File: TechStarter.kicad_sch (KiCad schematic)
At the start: 28 parts, among them J1 Conn_01x04_Socket, J10 Conn_01x03_Socket, J11 Conn_01x03_Socket, J12 Conn_01x04_Pin, J2 Conn_01x04_Socket, J5 Conn_01x03_Socket, J7 Conn_01x03_Socket, J8 Conn_01x03_Socket, J9 Conn_01x03_Socket, U1 STM32F446RETx, U2 TMC2209-LA, U3 TMC2209-LA, U5 MX25L3233FM1

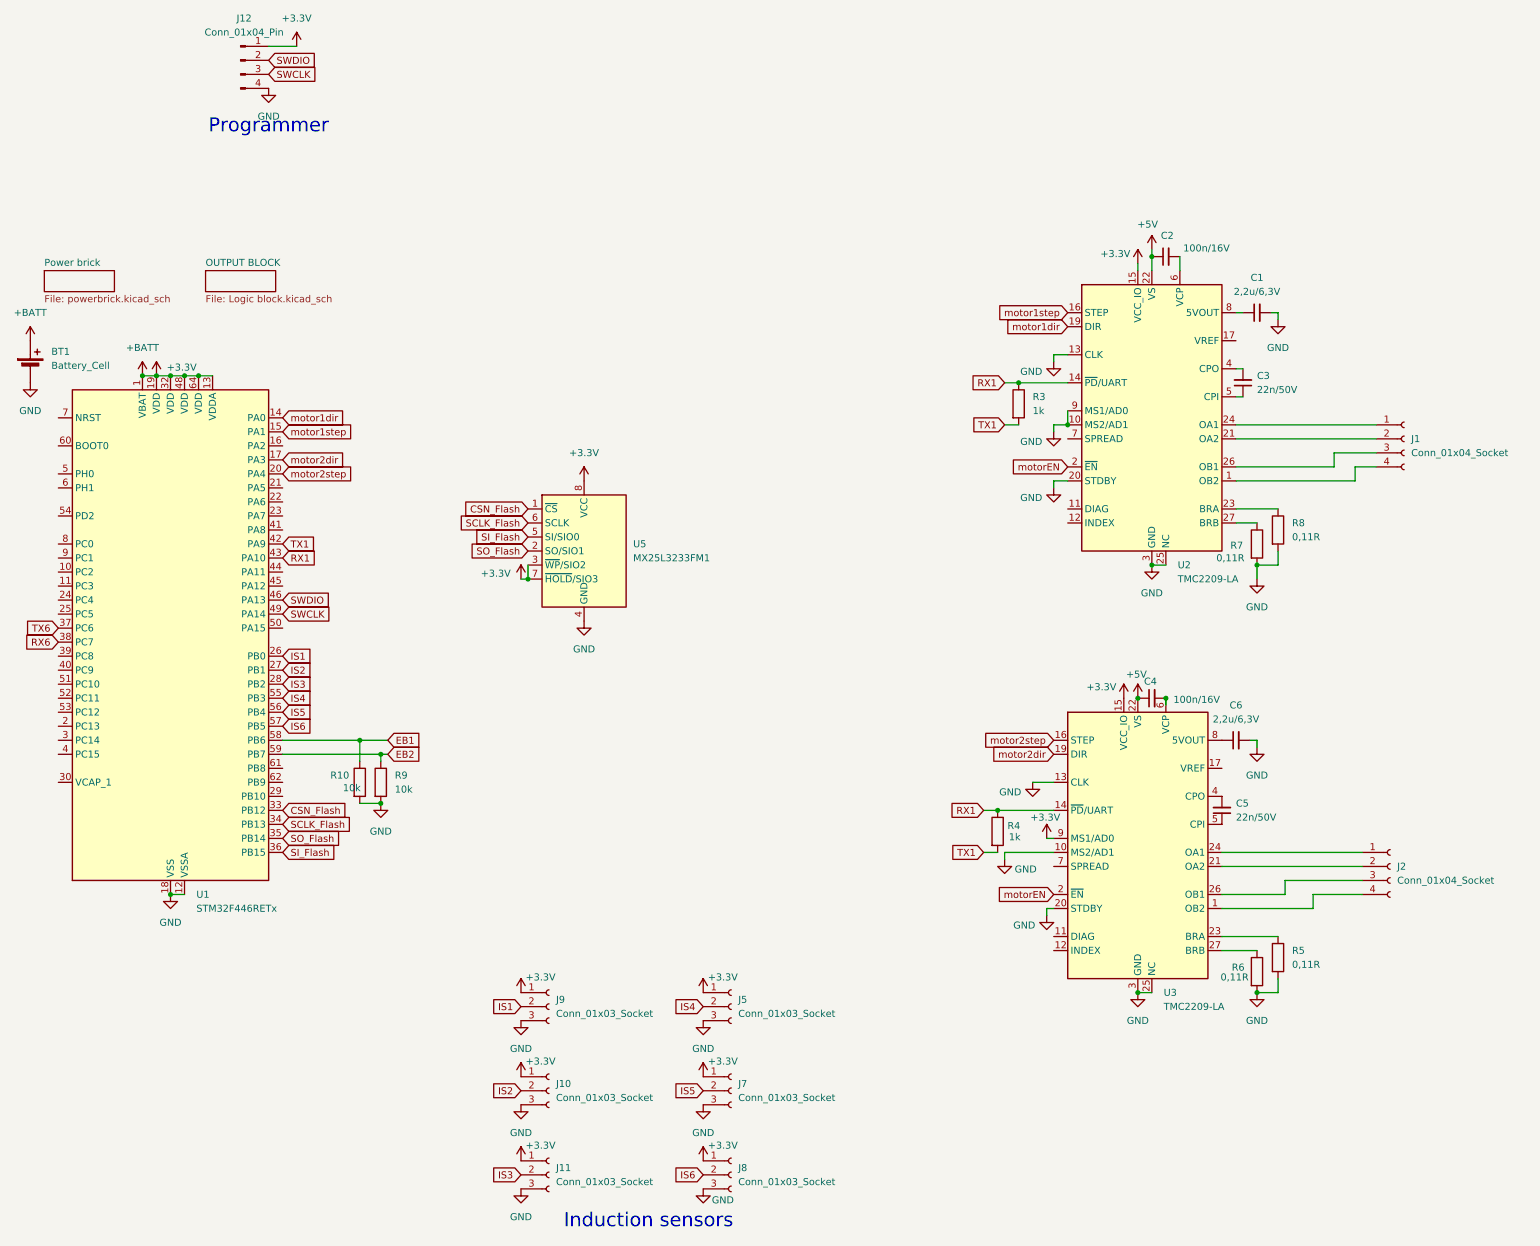
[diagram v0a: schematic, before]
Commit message: Board
started board ...
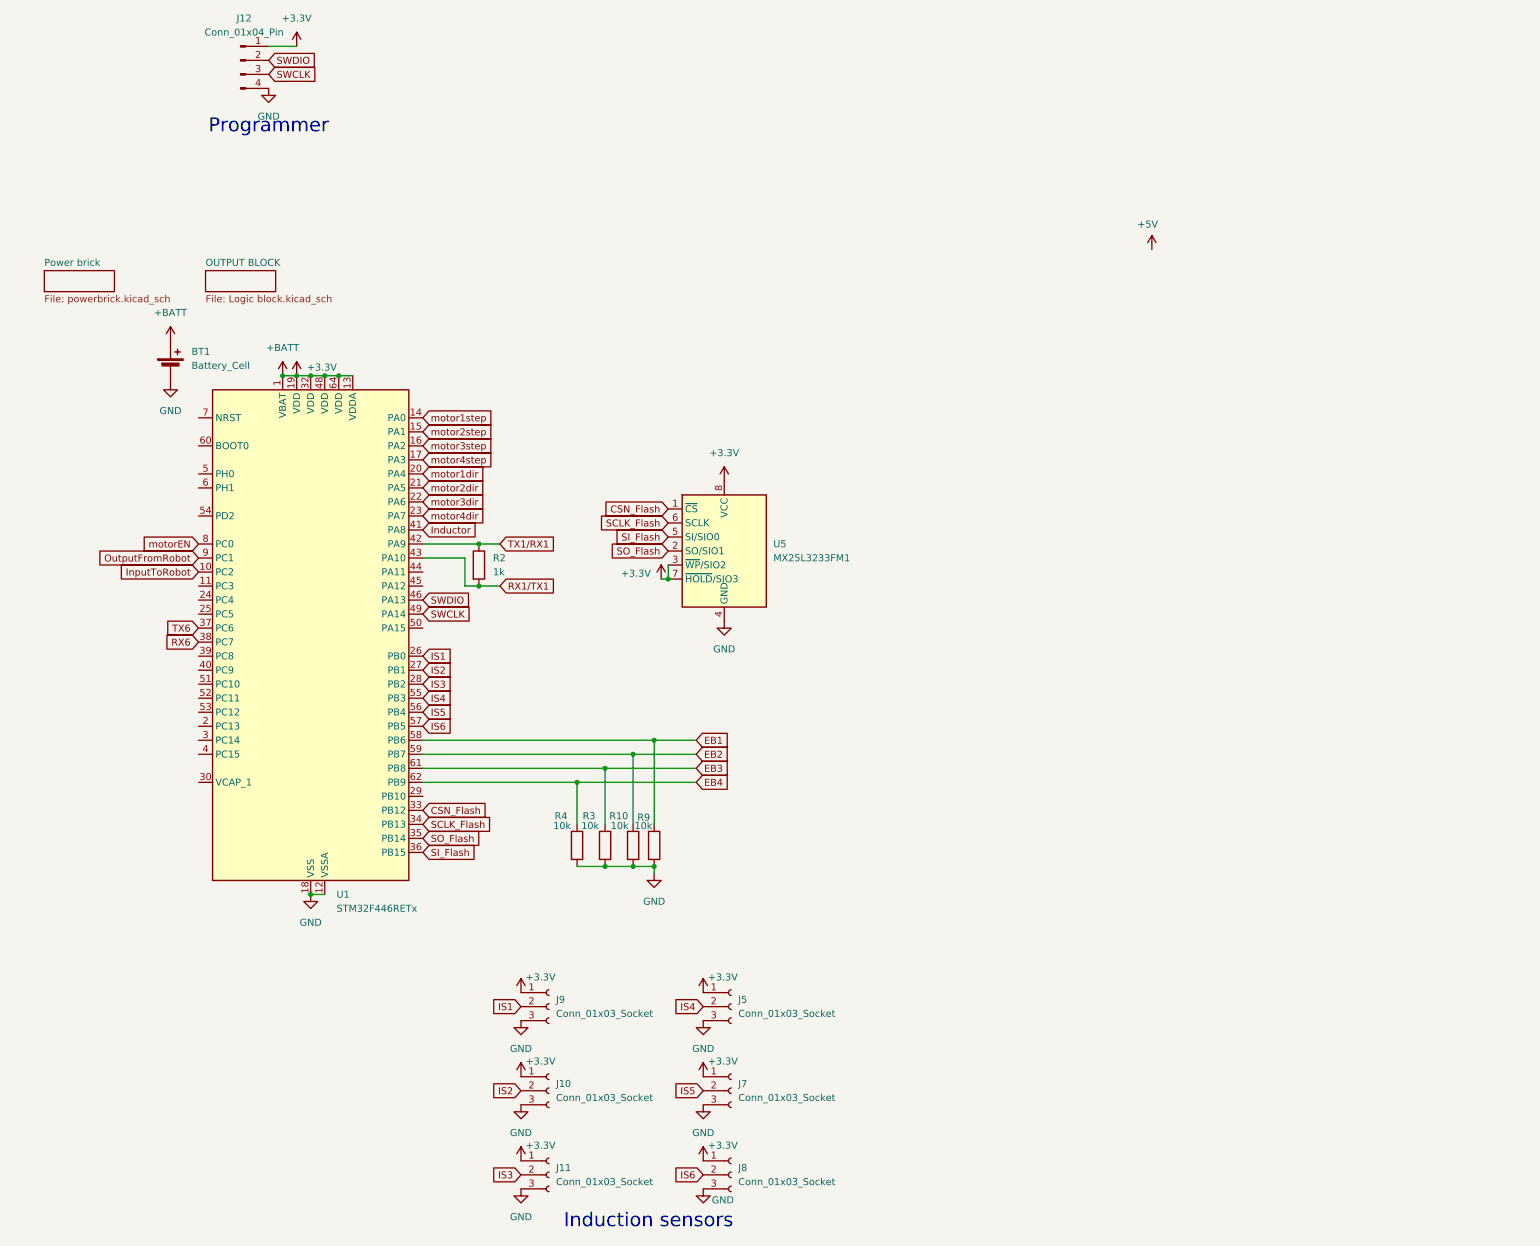
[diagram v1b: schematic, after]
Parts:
- removed C1: 2,2u/6,3V, Connector_JST:JST_XH_S3B-XH-A_1x03_P2.50mm_Horizontal, symbol Device:C_Small
- removed C2, C4: 100n/16V, symbol Device:C_Small
- removed C3, C5: 22n/50V, symbol Device:C_Small
- removed C6: 2,2u/6,3V, symbol Device:C_Small
- removed J1, J2: Conn_01x04_Socket, symbol Connector:Conn_01x04_Socket
- removed R5, R6, R7, R8: 0,11R, symbol Device:R
- removed U2, U3: TMC2209-LA, Package_DFN_QFN:VQFN-28-1EP_5x5mm_P0.5mm_EP3.7x3.7mm_ThermalVias, symbol Driver_Motor:TMC2209-LA
- added R2: 1k, Resistor_SMD:R_0603_1608Metric, symbol Device:R
- R10, R9: footprint (none) -> Resistor_SMD:R_0603_1608Metric
- R3, R4: value 1k -> 10k; footprint (none) -> Resistor_SMD:R_0603_1608Metric
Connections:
- net EB1: now also R9.1; no longer R10.1
- net EB2: now also R10.1; no longer R9.1
- net GND: now also R3.2, R4.2
- net motor1dir: now also U1.20 (PA4); no longer U1.14 (PA0)
- net motor1step: now also U1.14 (PA0); no longer U1.15 (PA1)
- net motor2dir: now also U1.21 (PA5); no longer U1.17 (PA3)
- net motor2step: now also U1.15 (PA1); no longer U1.20 (PA4)
- net motorEN: now also U1.8 (PC0)
- net InputToRobot: now reaches U1.10 (PC2)
- net motor3step: now reaches U1.16 (PA2)
- net motor3dir: now reaches U1.22 (PA6)
- net motor4dir: now reaches U1.23 (PA7)
- net Inductor: now reaches U1.41 (PA8)
- net EB3: now reaches U1.61 (PB8)
- net EB3: now also R3.1
- net EB4: now reaches U1.62 (PB9)
- net EB4: now also R4.1
- net OutputFromRobot: now reaches U1.9 (PC1)
- removed net RX1: R3.1, R4.1, U1.43 (PA10)
- removed net TX1: R3.2, R4.2, U1.42 (PA9)
- new net RX1/TX1: R2.2, U1.43 (PA10)
- new net TX1/RX1: R2.1, U1.42 (PA9)
- new net motor4step: U1.17 (PA3)
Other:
- moved on the sheet: BT1, R10, R9, U1, U5
